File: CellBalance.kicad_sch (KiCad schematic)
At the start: 8 parts, among them Q1 GSF3400

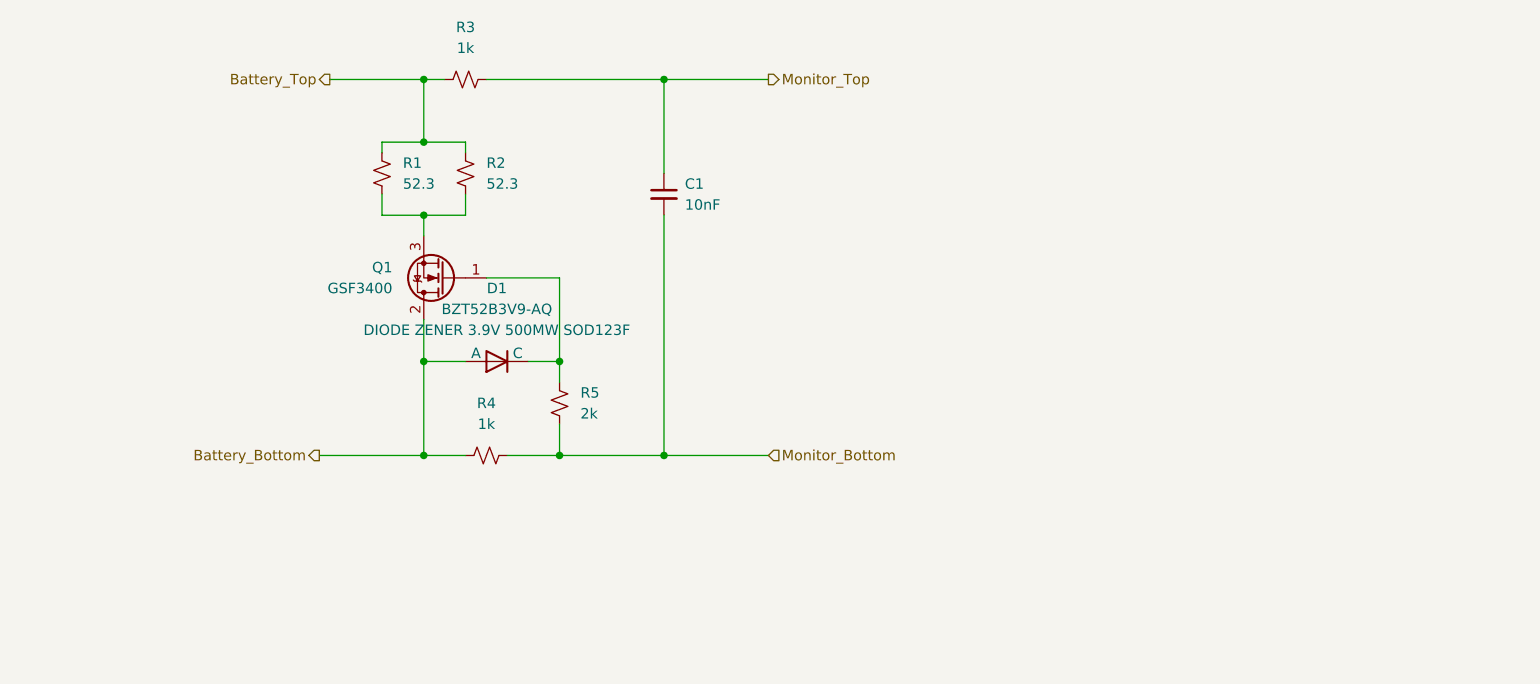
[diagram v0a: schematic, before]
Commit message: mostly done afe ic
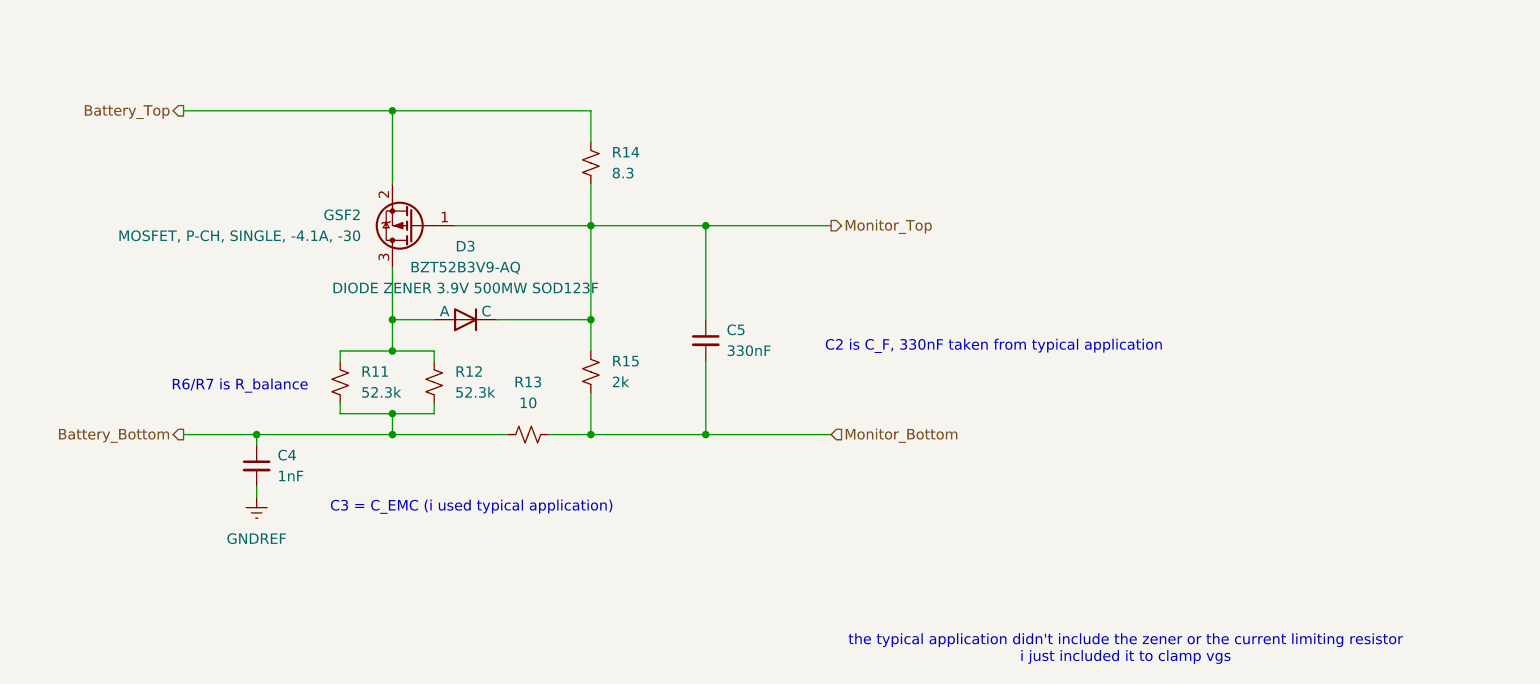
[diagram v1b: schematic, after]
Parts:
- removed C1: 10nF, symbol Device:C_Small
- removed D1: BZT52B3V9-AQ, footprints:P35_SOD-123F, symbol symbols:Diode
- removed Q1: GSF3400, Package_TO_SOT_SMD:SOT-23-3, symbol symbols:GSF3400
- removed R1, R2: 52.3, symbol Device:R_Small_US
- removed R3, R4: 1k, symbol Device:R_Small_US
- removed R5: 2k, symbol Device:R_Small_US
- added C4: 1nF, symbol Device:C_Small
- added C5: 330nF, symbol Device:C_Small
- added D3: BZT52B3V9-AQ, footprints:P35_SOD-123F, symbol symbols:Diode
- added GSF2: MOSFET, P-CH, SINGLE, -4.1A, -30, Package_TO_SOT_SMD:SOT-23-3, symbol symbols:GSF0304
- added R11, R12: 52.3k, symbol Device:R_Small_US
- added R13: 10, symbol Device:R_Small_US
- added R14: 8.3, symbol Device:R_Small_US
- added R15: 2k, symbol Device:R_Small_US
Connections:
- net Battery_Bottom: now also C4.1, R11.2, R12.2, R13.1
- net Battery_Top: now also GSF2.2 (S), R14.2
- net Monitor_Bottom: now also C5.2, R13.2, R15.1
- net Monitor_Top: now also C5.1, D3.2 (C), GSF2.1 (G), R14.1, R15.2
- new net: D3.1 (A), GSF2.3 (D), R11.1, R12.1
- new net GNDREF: C4.2
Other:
- note added: "C2 is C_F, 330nF taken from typical application"
- note added: "C3 = C_EMC (i used typical application)"
- note added: "R6/R7 is R_balance"
- note added: "the typical application didn't include the zener or the current limiting resistor i just included it to clamp vgs"
